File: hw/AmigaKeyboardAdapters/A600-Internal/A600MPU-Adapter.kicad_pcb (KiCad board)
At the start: 2 copper layers, 33 x 29.2 mm, 9 parts, among them P1 CONN_02X03, P2 CONN_01X03, U1 6571R4_PLCC44_MPUKEY_REV

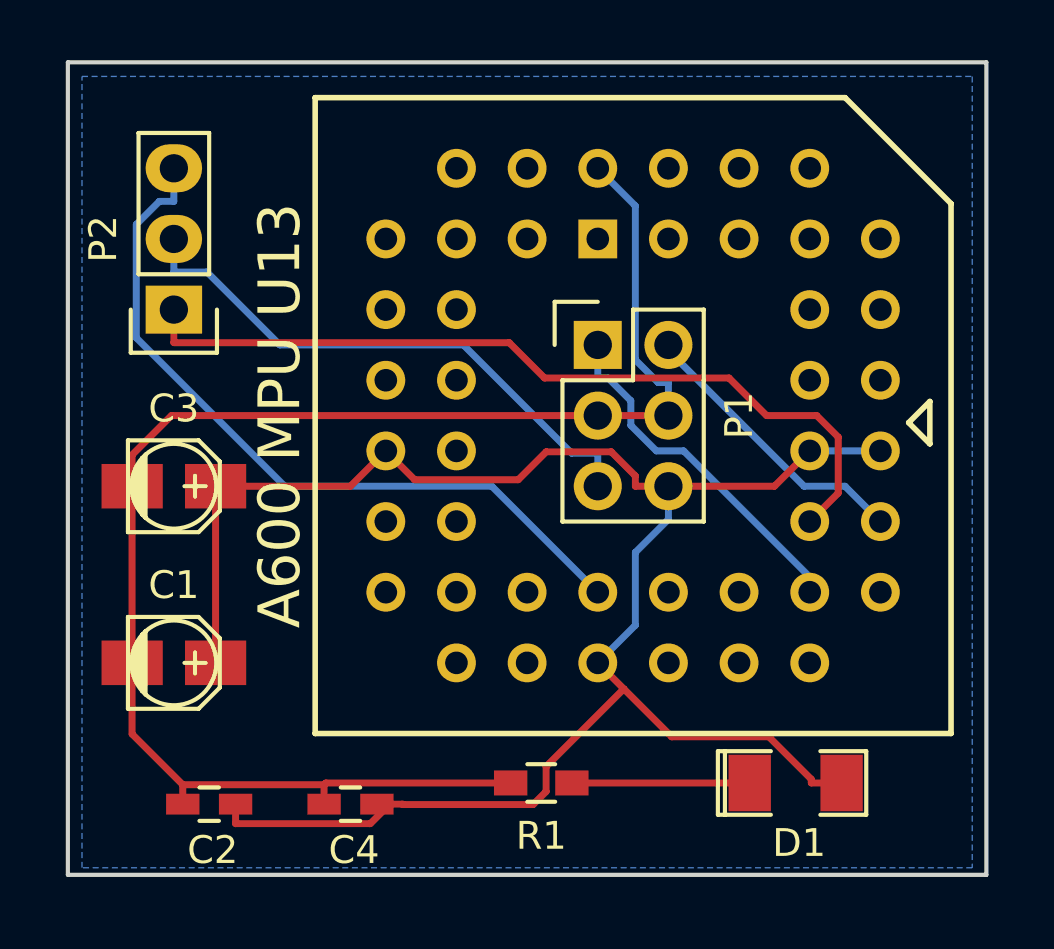
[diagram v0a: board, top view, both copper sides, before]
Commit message: From KiCAD 4 to KiCAD 5
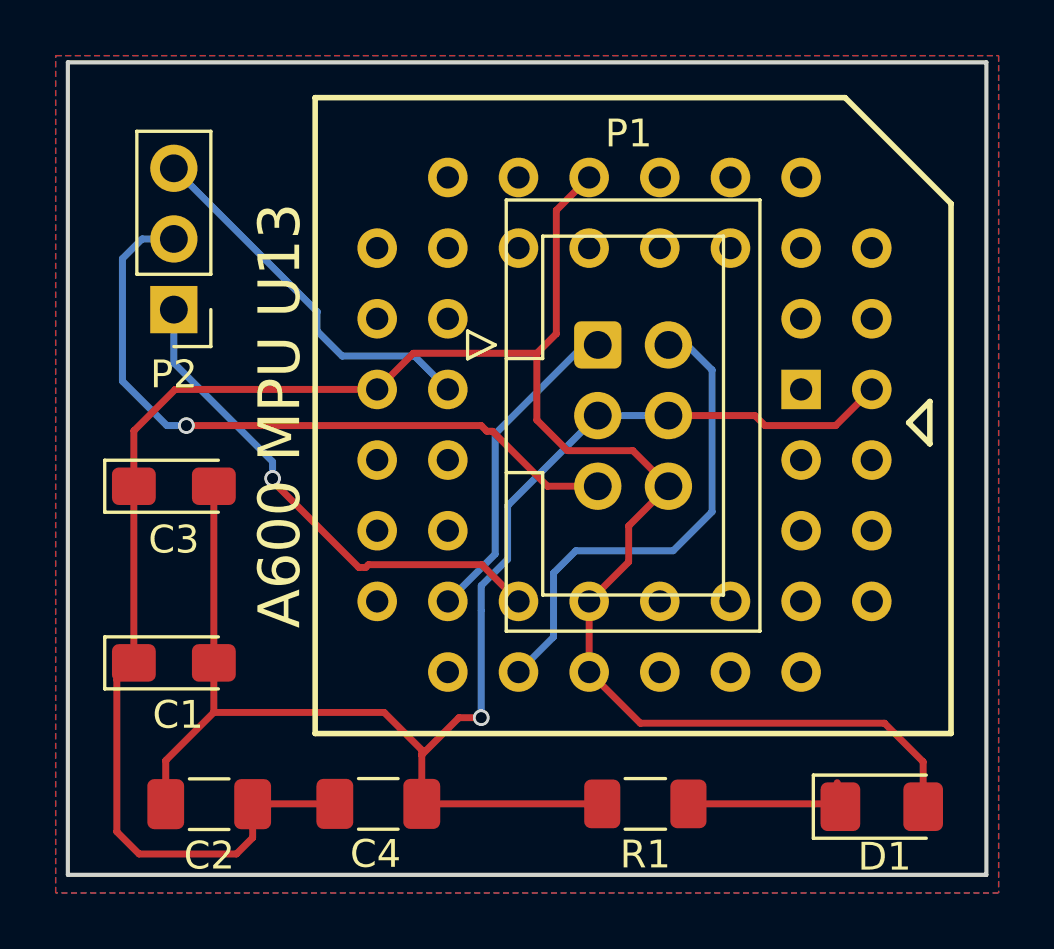
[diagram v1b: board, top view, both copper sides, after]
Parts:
- C1, C3: footprint Capacitors_SMD:c_elec_3x5.3 -> Capacitor_Tantalum_SMD:CP_EIA-3216-12_Kemet-S_Pad1.58x1.35mm_HandSolder
- C2, C4: footprint Capacitors_SMD:C_0603_HandSoldering -> Capacitor_SMD:C_1206_3216Metric_Pad1.33x1.80mm_HandSolder
- D1: value Led_Small -> RED; footprint SMD_Packages:SMD-1206_Pol -> LED_SMD:LED_1206_3216Metric_Pad1.42x1.75mm_HandSolder
- P1: footprint Pin_Headers:Pin_Header_Straight_2x03 -> Connector_IDC:IDC-Header_2x03_P2.54mm_Vertical
- P2: footprint Pin_Headers:Pin_Header_Straight_1x03 -> Connector_PinHeader_2.54mm:PinHeader_1x03_P2.54mm_Vertical
- R1: value 330 -> 330R; footprint Resistors_SMD:R_0603_HandSoldering -> Resistor_SMD:R_1206_3216Metric_Pad1.30x1.75mm_HandSolder
- U1: footprint Sockets:PLCC44 -> RetroBitLab:PLCC-44_THT-Socket_3D
- moved U1 6.11 mm to (168.6, 103.2), turned to 90 degrees
- moved R1 3.82 mm to (163.0, 118.1)
- moved D1 3.21 mm to (171.5, 118.2)
- moved C4 1.00 mm to (153.4, 118.1), turned to 0 degrees
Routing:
- net ~RST: track 27.3 -> 13.6 mm
- net ~TRESET: track 29.9 -> 18.4 mm, vias 0 -> 1
- net VCC: track 68.6 -> 78.0 mm
- net KBD_DATA: track 10.4 -> 17.7 mm
- net KBD_RESET: track 20.3 -> 25.2 mm, vias 0 -> 1
- net GND: track 55.9 -> 54.4 mm, vias 0 -> 1
- net KBD_CLOCK: track 12.8 -> 11.7 mm
- net Net-(D1-Pad1): track 6.39 -> 5.52 mm
- added copper zone on F.Cu, net GND
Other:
- rule pad_to_mask_clearance: 0.2 -> 0
- board text added: "designed by R.G.2018/2022"
- board text removed: "designed by R.G.2018"
